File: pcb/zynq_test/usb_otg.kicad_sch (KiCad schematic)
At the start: 18 parts, among them J1001 Conn_01x02, J1002 USB_A, U1001 DSC1001CI2-026, U1002 TUSB1210-Q1, U1003 AP22816AKBWT, U1004 ESD8104

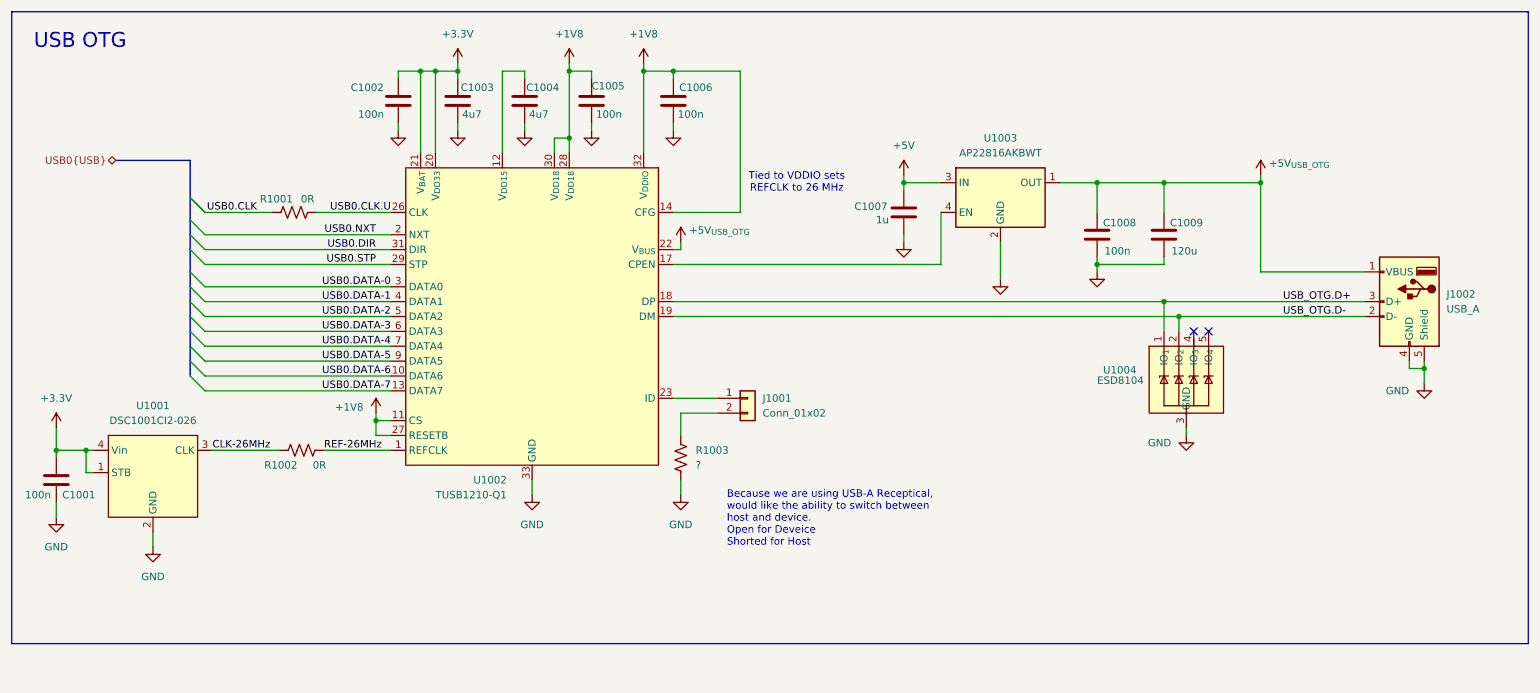
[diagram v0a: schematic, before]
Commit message: Finished Power Supply
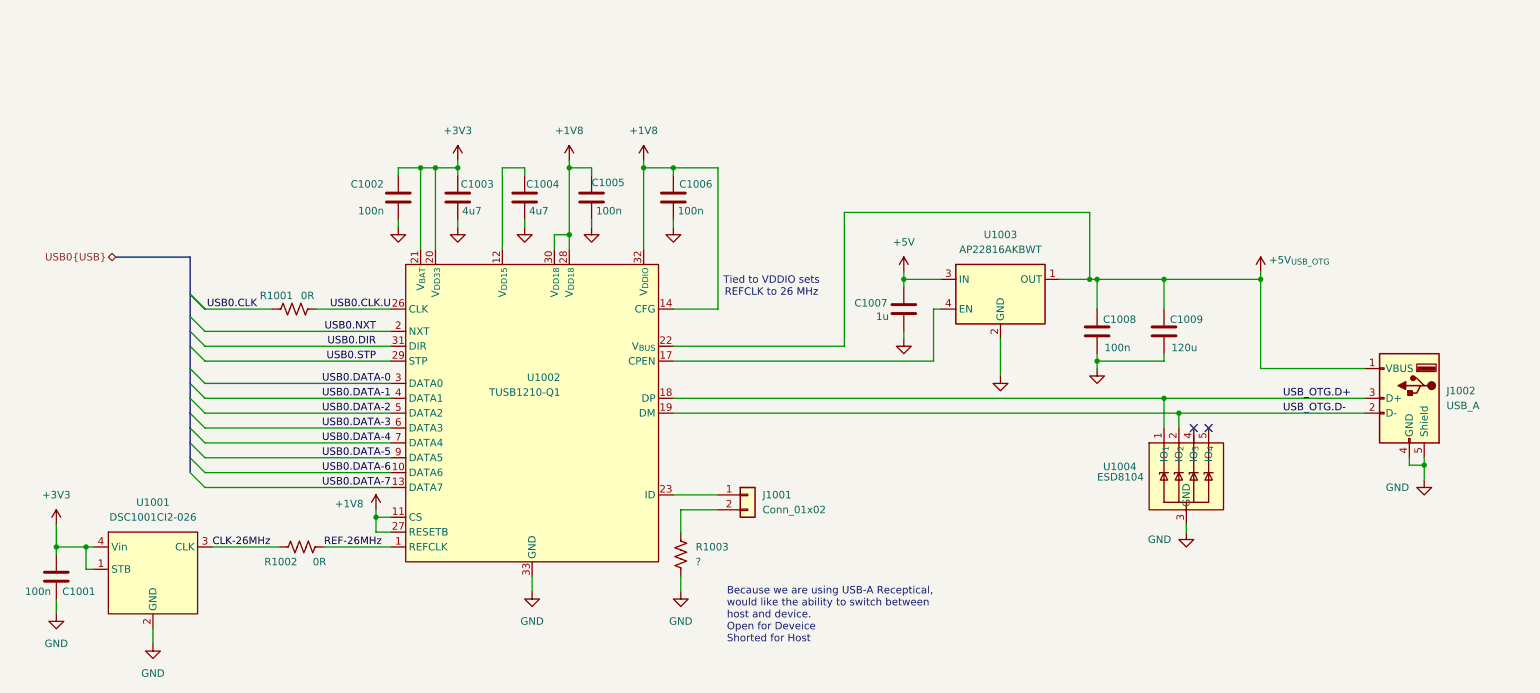
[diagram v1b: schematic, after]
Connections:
- net +3.3V renamed +3V3
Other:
- note removed: "USB OTG"
- title: (none) -> USB OTG
- moved on the sheet: C1001, C1002, C1003, C1004, C1005, C1006, C1007, C1008, C1009, J1001, J1002, R1001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
